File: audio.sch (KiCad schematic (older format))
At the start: 1 part, among them U1 DFR0299

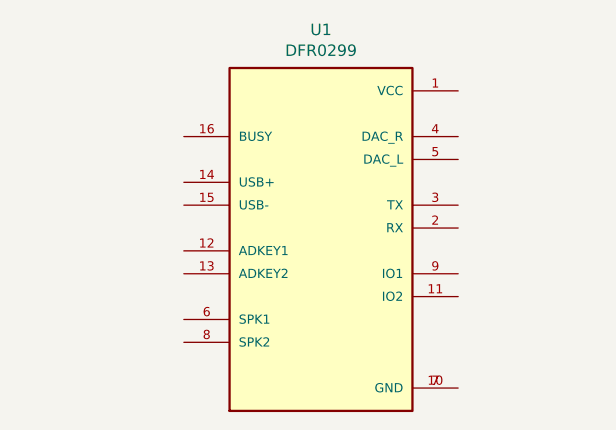
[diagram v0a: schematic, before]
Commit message: end of day save
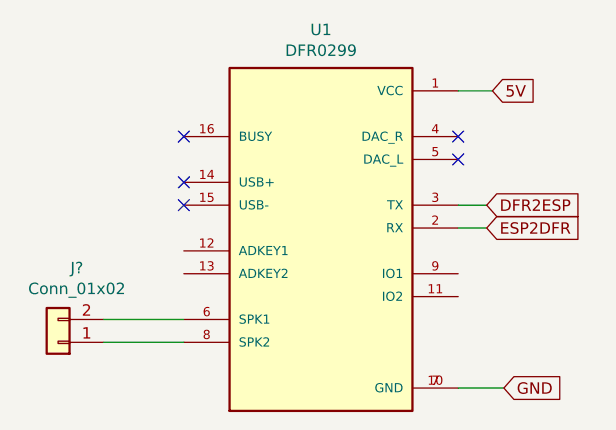
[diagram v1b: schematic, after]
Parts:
- added J?: Conn_01x02, Connector_JST:JST_XH_B2B-XH-A_1x02_P2.50mm_Vertical, symbol Connector_Generic:Conn_01x02
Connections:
- net 5V: now reaches U1.1 (VCC)
- net GND: now reaches U1.10 (GND), U1.7 (GND)
- net ESP2DFR: now reaches U1.2 (RX)
- net DFR2ESP: now reaches U1.3 (TX)
- net at U1.6 (SPK1): now also J?.2 (Pin_2)
- net at U1.8 (SPK2): now also J?.1 (Pin_1)
- no-connect marks 0 -> 5
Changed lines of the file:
@@
 	1    0    0    -1
 $EndComp
+$Comp
+L Connector_Generic:Conn_01x02 J?
+U 1 1 5FC6CA52
+P 4975 2850
+F 0 "J?" H 4893 2525 50  0000 C CNN
+F 1 "Conn_01x02" H 4893 2616 50  0000 C CNN
+F 2 "Connector_JST:JST_XH_B2B-XH-A_1x02_P2.50mm_Vertical" H 4975 2850 50  0001 C CNN
+F 3 "~" H 4975 2850 50  0001 C CNN
+	1    4975 2850
+	-1   0    0    1
+$EndComp
+Wire Wire Line
+	5175 2750 5525 2750
+Wire Wire Line
+	5175 2850 5525 2850
+Text GLabel 6925 3050 2    50   Input ~ 0
+GND
+Wire Wire Line
+	6725 3050 6925 3050
+Text GLabel 6875 1750 2    50   Input ~ 0
+5V
+Wire Wire Line
+	6725 1750 6875 1750
+NoConn ~ 6725 1950
+NoConn ~ 6725 2050
+Text GLabel 6850 2350 2    50   Input ~ 0
+ESP2DFR
+Text GLabel 6850 2250 2    50   Input ~ 0
+DFR2ESP
+Wire Wire Line
+	6725 2250 6850 2250
+Wire Wire Line
+	6725 2350 6850 2350
+NoConn ~ 5525 2150
+NoConn ~ 5525 1950
+NoConn ~ 5525 2250
 $EndSCHEMATC
